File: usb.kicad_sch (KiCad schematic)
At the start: 35 parts, among them J1 USB_C_Receptacle_USB2.0, U32 93LC46B, U33 FT2232H, Y1 ABM10-167-12.000MHZ-T3

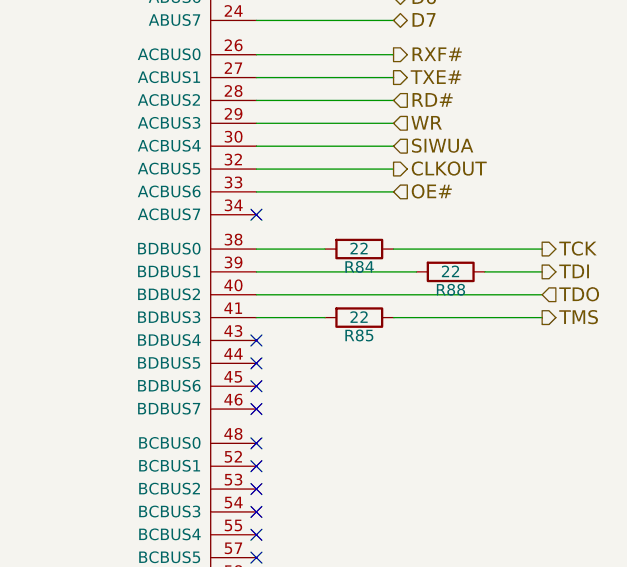
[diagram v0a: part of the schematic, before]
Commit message: clock buffer and txco source is changed. Clock is clipped sin and fanout says cmos square out but it is better anyways. Also traces are 50 ohm as well. Copper pours other minor thinks are changed as well
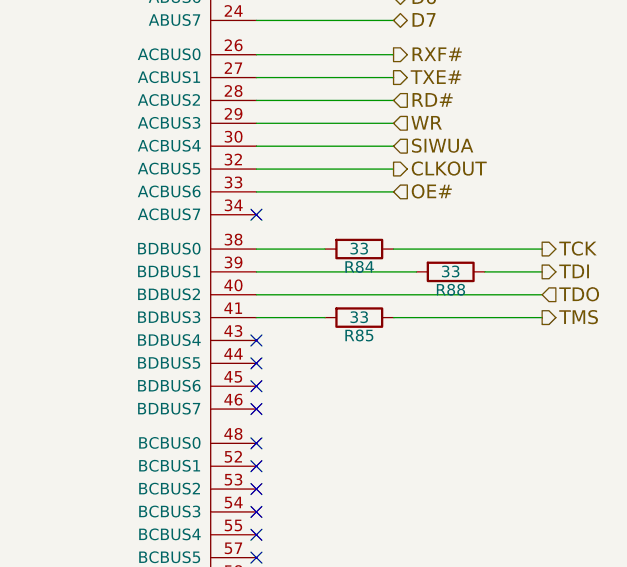
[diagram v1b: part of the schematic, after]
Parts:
- R84, R85, R88: value 22 -> 33
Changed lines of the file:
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@@
 			)
 		)
-		(property "Value" "22"
+		(property "Value" "33"
 			(at 203.2 101.6 90)
 			(effects
@@
 			)
 		)
-		(property "Value" "22"
+		(property "Value" "33"
 			(at 213.36 104.14 90)
 			(effects
@@
 			)
 		)
-		(property "Value" "22"
+		(property "Value" "33"
 			(at 203.2 109.22 90)
 			(effects

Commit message: I increased the gap between voltage pours and also corrected signals cutting copper pour. Also not connected gnd occured in some layers are corrected with no copper zoens
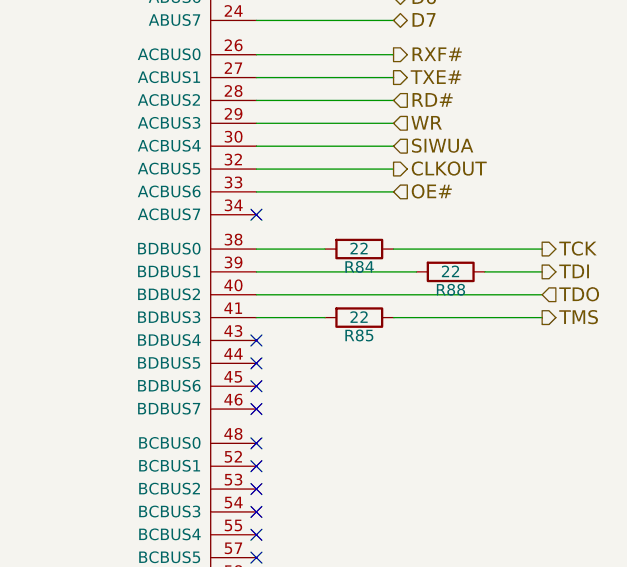
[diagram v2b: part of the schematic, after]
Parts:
- R84, R85, R88: value 33 -> 22
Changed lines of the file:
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@@
 			)
 		)
-		(property "Value" "33"
+		(property "Value" "22"
 			(at 203.2 101.6 90)
 			(effects
@@
 			)
 		)
-		(property "Value" "33"
+		(property "Value" "22"
 			(at 213.36 104.14 90)
 			(effects
@@
 			)
 		)
-		(property "Value" "33"
+		(property "Value" "22"
 			(at 203.2 109.22 90)
 			(effects
